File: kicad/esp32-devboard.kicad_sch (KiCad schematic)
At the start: 19 parts, among them J1 Conn_01x20, J2 Conn_01x20, J3 USB_C_Receptacle_USB2.0_16P, SW1 SW_Push, SW2 SW_Push, U1 ESP32-S3-WROOM-1, U2 LD1117S33TR_SOT223

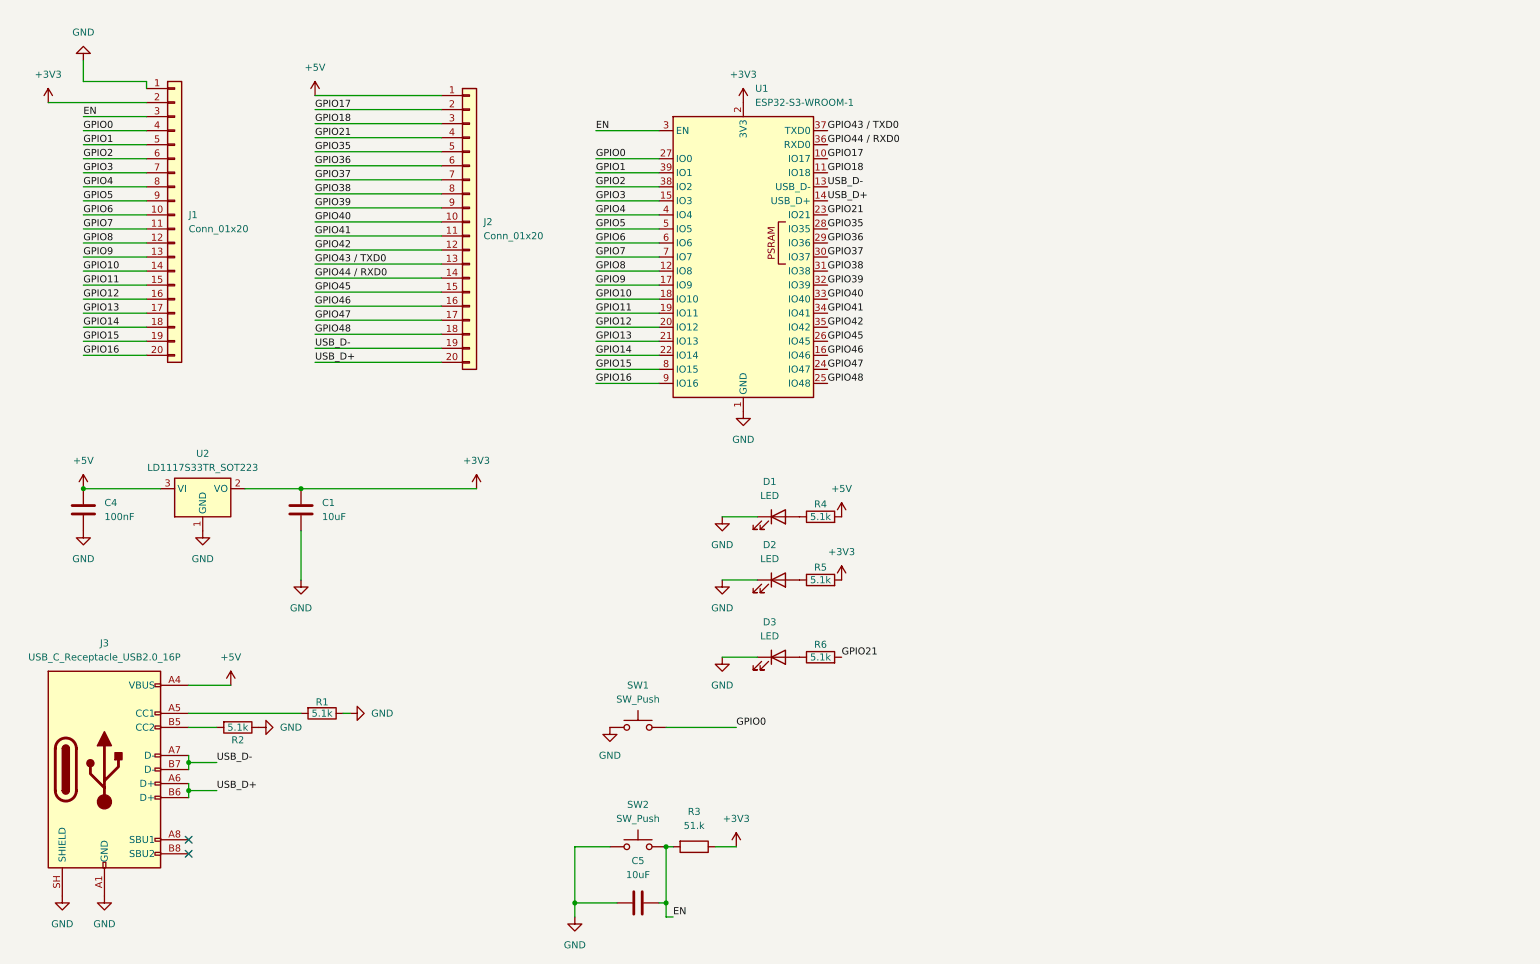
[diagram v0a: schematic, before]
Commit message: added
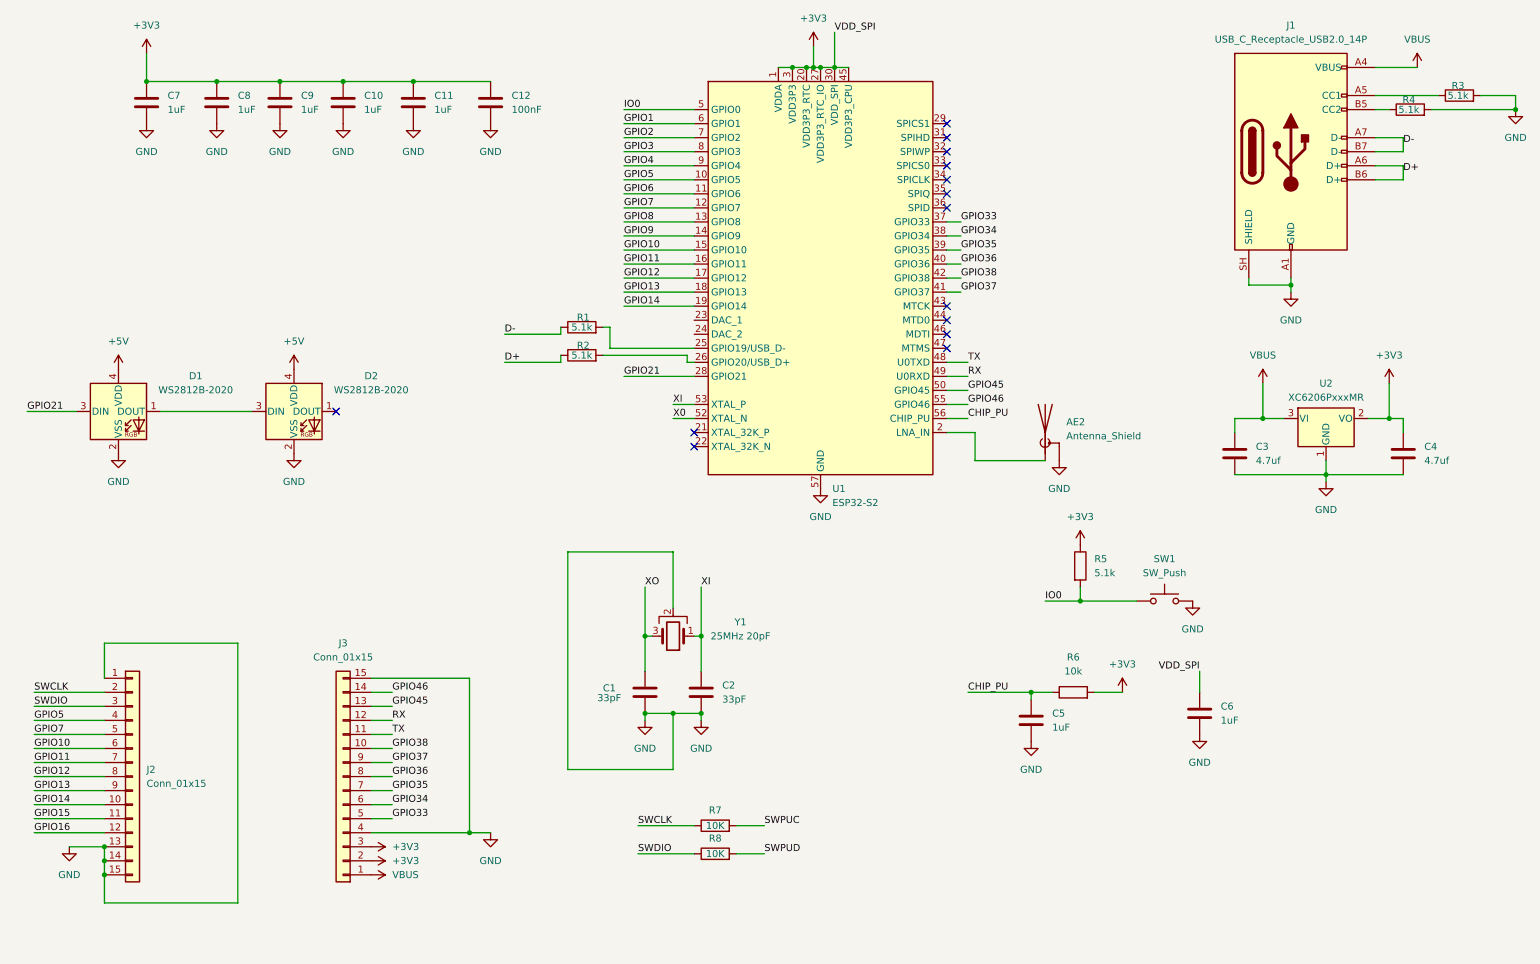
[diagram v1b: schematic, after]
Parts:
- removed D1, D2, D3: LED, LED_THT:LED_D3.0mm, symbol Device:LED
- removed J1, J2: Conn_01x20, Connector_PinHeader_2.54mm:PinHeader_1x20_P2.54mm_Vertical, symbol Connector_Generic:Conn_01x20
- removed J3: USB_C_Receptacle_USB2.0_16P, Connector_USB:USB_C_Receptacle_GCT_USB4105-xx-A_16P_TopMnt_Horizontal, symbol Connector:USB_C_Receptacle_USB2.0_16P
- removed SW2: SW_Push, Button_Switch_Keyboard:SW_Cherry_MX_1.00u_PCB, symbol Switch:SW_Push
- removed U1: ESP32-S3-WROOM-1, RF_Module:ESP32-S3-WROOM-1, symbol RF_Module:ESP32-S3-WROOM-1
- removed U2: LD1117S33TR_SOT223, Package_TO_SOT_SMD:SOT-223-3_TabPin2, symbol Regulator_Linear:LD1117S33TR_SOT223
- added AE2: Antenna_Shield, RF_Antenna:Texas_SWRA117D_2.4GHz_Left, symbol Device:Antenna_Shield
- added C10, C11, C6, C7, C8, C9: 1uF, Capacitor_SMD:C_0402_1005Metric, symbol Device:C
- added C12: 100nF, Capacitor_SMD:C_0402_1005Metric, symbol Device:C
- added C2: 33pF, Capacitor_SMD:C_0402_1005Metric, symbol Device:C
- added C3: 4.7uf, Capacitor_SMD:C_0402_1005Metric, symbol Device:C
- added D1, D2: WS2812B-2020, LED_SMD:LED_WS2812B-2020_PLCC4_2.0x2.0mm, symbol LED:WS2812B-2020
- added J1: USB_C_Receptacle_USB2.0_14P, Connector_USB:USB_C_Receptacle_HRO_TYPE-C-31-M-12, symbol Connector:USB_C_Receptacle_USB2.0_14P
- added J2, J3: Conn_01x15, Connector_PinHeader_2.54mm:PinHeader_1x15_P2.54mm_Vertical, symbol Connector_Generic:Conn_01x15
- added R7, R8: 10K, Resistor_SMD:R_0402_1005Metric, symbol Device:R
- added U1: ESP32-S2, Package_DFN_QFN:QFN-56-1EP_7x7mm_P0.4mm_EP4x4mm, symbol MCU_Espressif:ESP32-S2
- added U2: XC6206PxxxMR, Package_TO_SOT_SMD:SOT-23-3, symbol Regulator_Linear:XC6206PxxxMR
- added Y1: 25MHz 20pF, Crystal:Crystal_SMD_2016-4Pin_2.0x1.6mm, symbol Device:Crystal_GND2
- C1: value 10uF -> 33pF; footprint Capacitor_SMD:C_1206_3216Metric -> Capacitor_SMD:C_0402_1005Metric
- C4: value 100nF -> 4.7uf; footprint Capacitor_SMD:C_1206_3216Metric -> Capacitor_SMD:C_0402_1005Metric
- C5: value 10uF -> 1uF; footprint Capacitor_SMD:C_1206_3216Metric -> Capacitor_SMD:C_0402_1005Metric
- R1, R2, R4, R5: footprint Resistor_SMD:R_1206_3216Metric -> Resistor_SMD:R_0402_1005Metric
- R3: value 51.k -> 5.1k; footprint Resistor_SMD:R_1206_3216Metric -> Resistor_SMD:R_0402_1005Metric
- R6: value 5.1k -> 10k; footprint Resistor_SMD:R_1206_3216Metric -> Resistor_SMD:R_0402_1005Metric
- SW1: footprint Button_Switch_Keyboard:SW_Cherry_MX_1.00u_PCB -> Button_Switch_THT:SW_PUSH_6mm
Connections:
- net EN is gone; now on net GND: C5.2, R3.2
- net GPIO0 is gone; now on net GND: SW1.2
- net +3V3: now also C4.1, R5.1, R6.2, C10.1, C11.1, C12.1, C6.1, C7.1, C8.1, C9.1, J3.2 (Pin_2), J3.3 (Pin_3), U1.1 (VDDA), U1.20 (VDD3P3_RTC), U1.27 (VDD3P3_RTC_IO), U1.3 (VDD3P3), U1.30 (VDD_SPI), U1.4 (VDD3P3), U1.45 (VDD3P3_CPU), U1.51 (VDDA), U1.54 (VDDA), U2.2 (VO); no longer C1.1, R3.1, R5.2
- net +5V: now also D1.4 (VDD), D2.4 (VDD); no longer C4.1, R4.2
- net GND: now also R4.2, AE2.2 (Shield), C10.2, C11.2, C12.2, C2.2, C3.2, C6.2, C7.2, C8.2, C9.2, D1.2 (VSS), D2.2 (VSS), J1.A1 (GND), J1.A12 (GND), J1.B1 (GND), J1.B12 (GND), J1.SH (SHIELD), J2.1 (Pin_1), J2.13 (Pin_13), J2.14 (Pin_14), J2.15 (Pin_15), J3.15 (Pin_15), J3.4 (Pin_4), U1.57 (GND), U2.1 (GND), Y1.2; no longer C5.1, R1.1, R2.1, SW1.1
- net GPIO1: now also U1.6 (GPIO1)
- net GPIO10: now also J2.6 (Pin_6), U1.15 (GPIO10)
- net GPIO11: now also J2.7 (Pin_7), U1.16 (GPIO11)
- net GPIO12: now also J2.8 (Pin_8), U1.17 (GPIO12)
- net GPIO13: now also J2.9 (Pin_9), U1.18 (GPIO13)
- net GPIO14: now also J2.10 (Pin_10), U1.19 (GPIO14)
- net GPIO15: now also J2.11 (Pin_11)
- net GPIO16: now also J2.12 (Pin_12)
- net GPIO2: now also U1.7 (GPIO2)
- net GPIO21: now also D1.3 (DIN), U1.28 (GPIO21); no longer R6.2
- net GPIO3: now also U1.8 (GPIO3)
- net GPIO35: now also J3.7 (Pin_7), U1.39 (GPIO35)
- net GPIO36: now also J3.8 (Pin_8), U1.40 (GPIO36)
- net GPIO37: now also J3.9 (Pin_9), U1.41 (GPIO37)
- net GPIO38: now also J3.10 (Pin_10), U1.42 (GPIO38)
- net GPIO4: now also U1.9 (GPIO4)
- net GPIO45: now also J3.13 (Pin_13), U1.50 (GPIO45)
- net GPIO46: now also J3.14 (Pin_14), U1.55 (GPIO46)
- net GPIO5: now also J2.4 (Pin_4), U1.10 (GPIO5)
- net GPIO6: now also U1.11 (GPIO6)
- net GPIO7: now also J2.5 (Pin_5), U1.12 (GPIO7)
- net GPIO8: now also U1.13 (GPIO8)
- net GPIO9: now also U1.14 (GPIO9)
- net at R4.1: now also J1.B5 (CC2)
- net at R1.2: now also U1.25 (GPIO19/USB_D-)
- net at R2.2: now also U1.26 (GPIO20/USB_D+)
- net CHIP_PU: now reaches R6.1
- net CHIP_PU: now also C5.1, U1.56 (CHIP_PU)
- new net: D1.1 (DOUT), D2.3 (DIN)
- new net: AE2.1 (A), U1.2 (LNA_IN)
- new net: J1.A5 (CC1), R3.1
- new net D+: J1.A6 (D+), J1.B6 (D+), R2.1
- new net D-: J1.A7 (D-), J1.B7 (D-), R1.1
- new net GPIO33: J3.5 (Pin_5), U1.37 (GPIO33)
- new net GPIO34: J3.6 (Pin_6), U1.38 (GPIO34)
- new net IO0: R5.2, SW1.1, U1.5 (GPIO0)
- new net RX: J3.12 (Pin_12), U1.49 (U0RXD)
- new net SWCLK: J2.2 (Pin_2), R7.1
- new net SWDIO: J2.3 (Pin_3), R8.1
- new net SWPUC: R7.2
- new net SWPUD: R8.2
- new net TX: J3.11 (Pin_11), U1.48 (U0TXD)
- new net VBUS: C3.1, J1.A4 (VBUS), J1.A9 (VBUS), J1.B4 (VBUS), J1.B9 (VBUS), J3.1 (Pin_1), U2.3 (VI)
- new net X0: U1.52 (XTAL_N)
- new net XI: C2.1, U1.53 (XTAL_P), Y1.1
- new net XO: C1.1, Y1.3
- no-connect marks 2 -> 14
